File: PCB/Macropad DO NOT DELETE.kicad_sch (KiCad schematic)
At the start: 9 parts, among them SW1 SW_Push, SW10 RotaryEncoder, SW2 SW_Push, SW3 SW_Push, SW4 SW_Push, SW5 SW_Push, SW9 RotaryEncoder, U1 MOUDLE-SEEEDUINO-XIAO, U2 ER_OLEDM0.91_1x-I2C

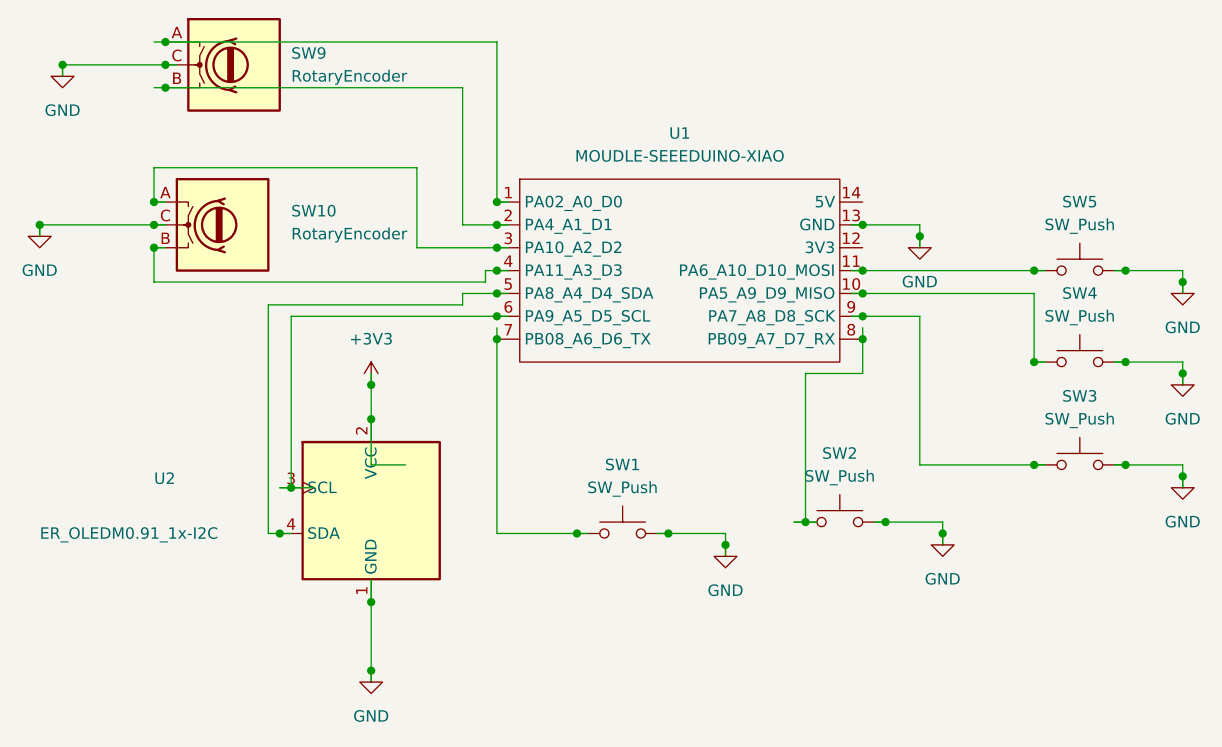
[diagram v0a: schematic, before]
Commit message: after rechecking
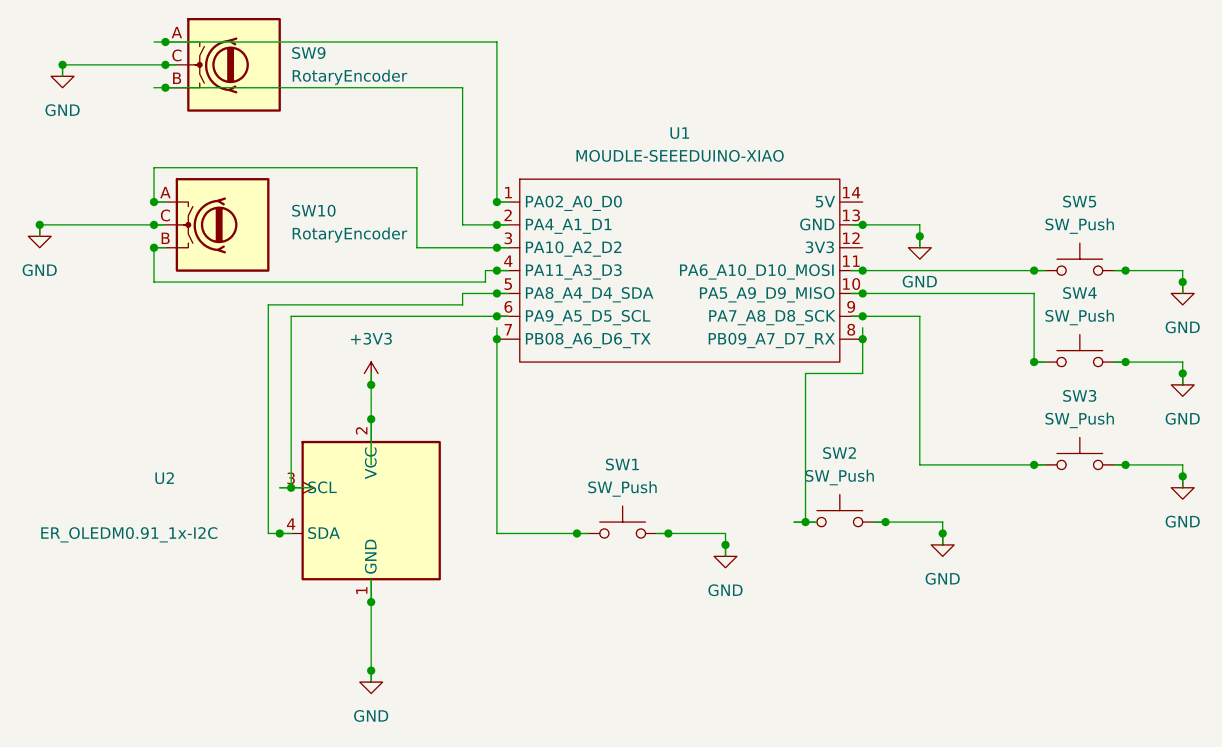
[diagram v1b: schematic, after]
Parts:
- SW1, SW2, SW3, SW4, SW5: footprint Button_Switch_THT:SW_PUSH_6mm -> Button_Switch_Keyboard:SW_Cherry_MX_1.00u_PCB
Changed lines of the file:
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@@
-	(wire
-		(pts
-			(xy 91.44 110.49) (xy 95.25 110.49)
-		)
-		(stroke
-			(width 0)
-			(type default)
-		)
-	)
 	(wire
 		(pts
@@
 			)
 		)
-		(property "Footprint" "Button_Switch_THT:SW_PUSH_6mm"
+		(property "Footprint" "Button_Switch_Keyboard:SW_Cherry_MX_1.00u_PCB"
 			(at 143.51 111.76 0)
 			(hide yes)
@@
 			)
 		)
-		(property "Footprint" "Button_Switch_THT:SW_PUSH_6mm"
+		(property "Footprint" "Button_Switch_Keyboard:SW_Cherry_MX_1.00u_PCB"
 			(at 170.18 105.41 0)
 			(hide yes)
@@
 			)
 		)
-		(property "Footprint" "Button_Switch_THT:SW_PUSH_6mm"
+		(property "Footprint" "Button_Switch_Keyboard:SW_Cherry_MX_1.00u_PCB"
 			(at 170.18 83.82 0)
 			(hide yes)
@@
 			)
 		)
-		(property "Footprint" "Button_Switch_THT:SW_PUSH_6mm"
+		(property "Footprint" "Button_Switch_Keyboard:SW_Cherry_MX_1.00u_PCB"
 			(at 170.18 93.98 0)
 			(hide yes)
@@
 			)
 		)
-		(property "Footprint" "Button_Switch_THT:SW_PUSH_6mm"
+		(property "Footprint" "Button_Switch_Keyboard:SW_Cherry_MX_1.00u_PCB"
 			(at 119.38 113.03 0)
 			(hide yes)
